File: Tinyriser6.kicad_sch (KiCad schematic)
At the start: 21 parts, among them J1 Bus_M.2_Socket_M, J2 Bus_PCI_Express_x16, J3 Conn_02x04_Odd_Even, J6 USB_A, J7 Conn_01x26_Pin, M1 Fan_4pin

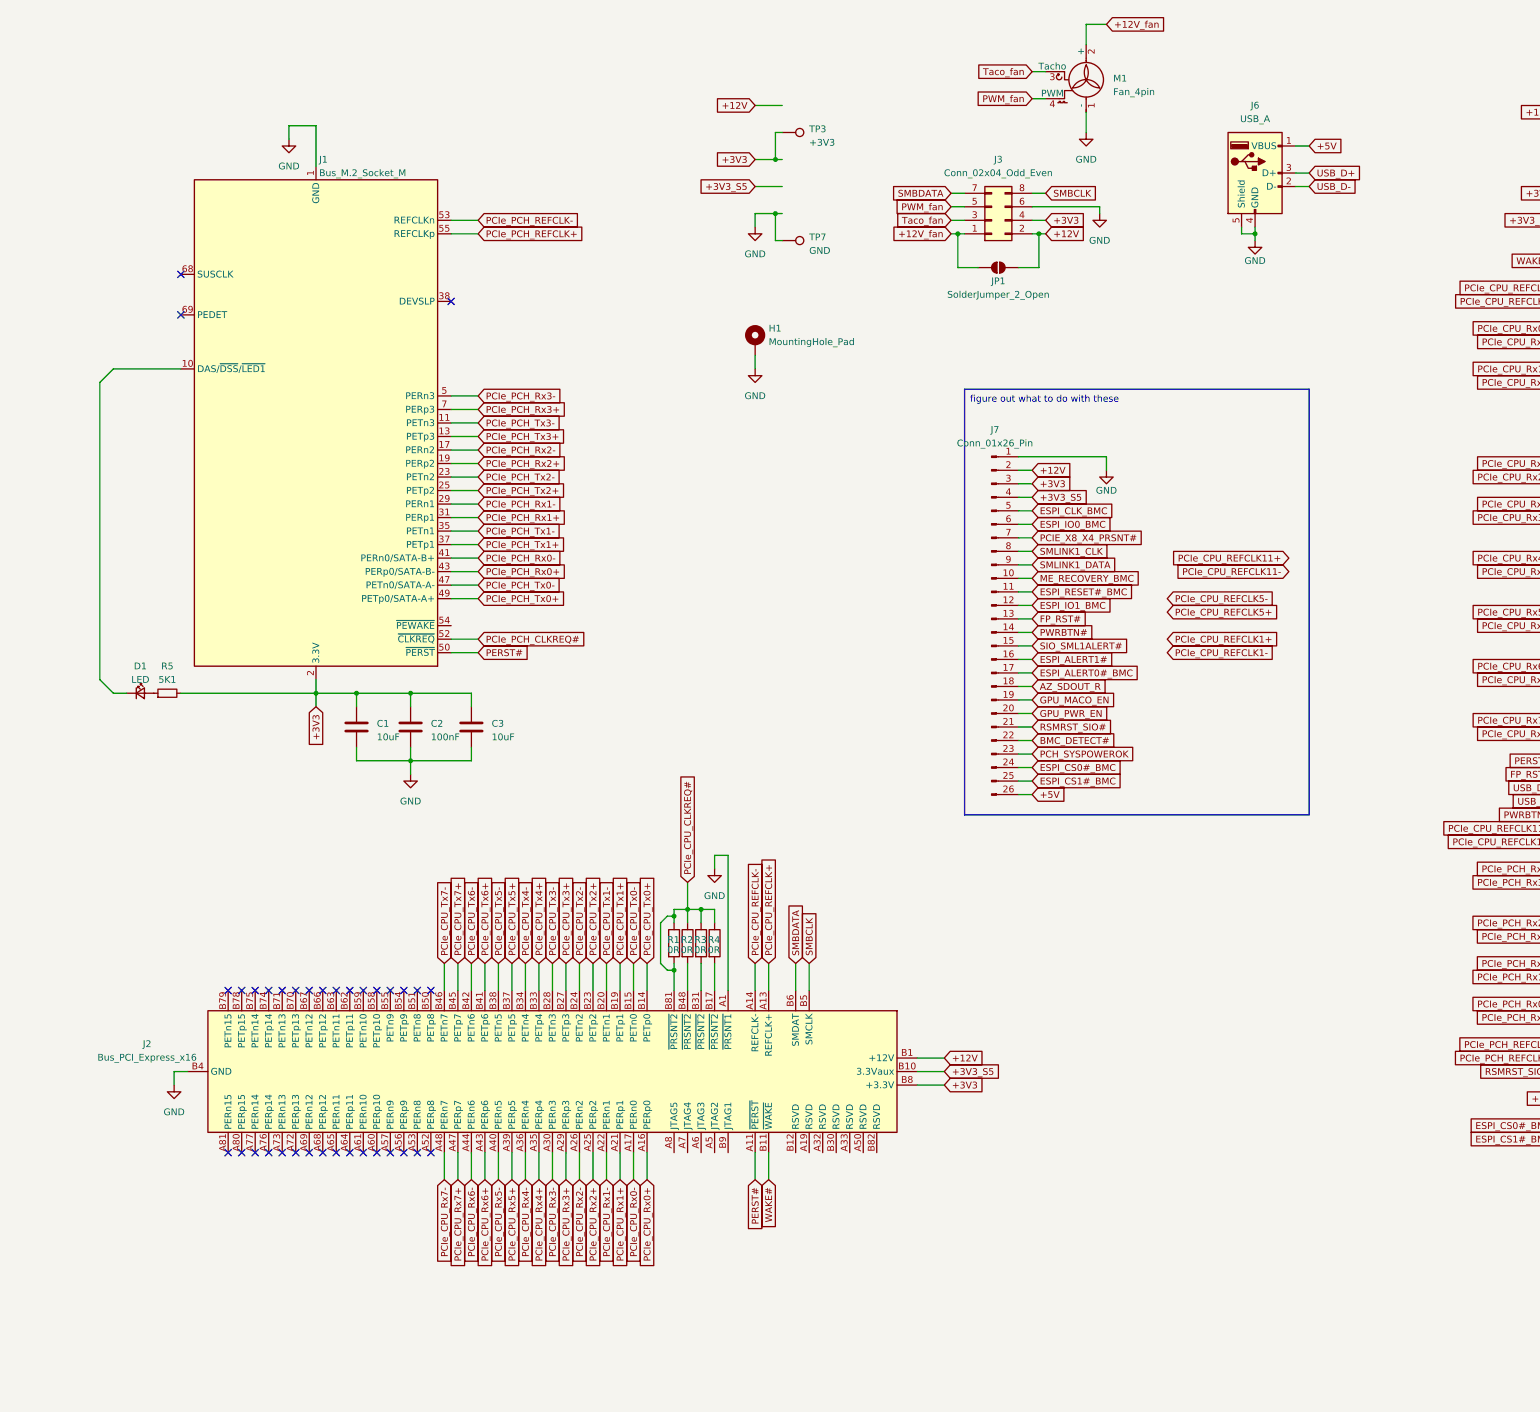
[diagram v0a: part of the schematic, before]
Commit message: Trying to figure out what to do with the random io
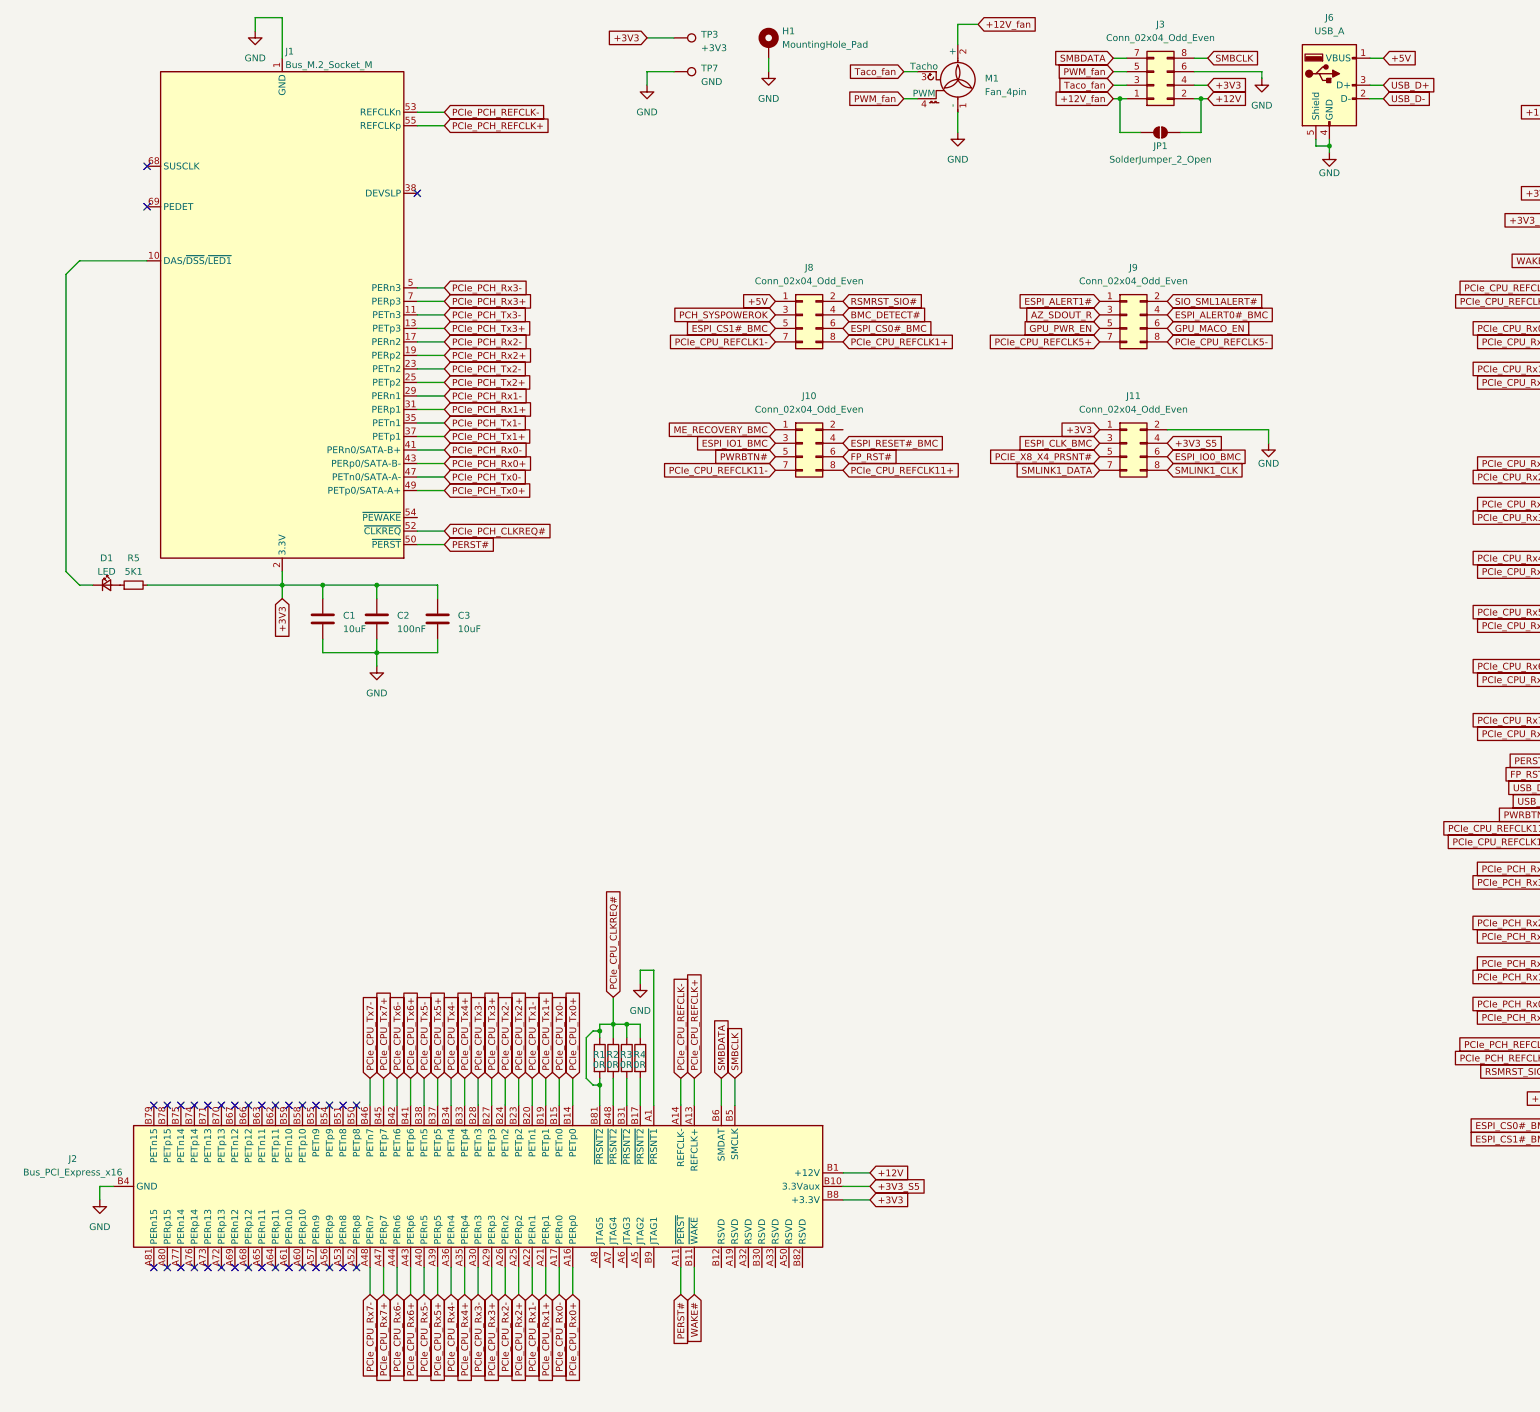
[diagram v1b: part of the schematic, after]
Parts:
- removed J7: Conn_01x26_Pin, Connector_PinHeader_2.00mm:PinHeader_2x13_P2.00mm_Vertical, symbol Connector:Conn_01x26_Pin
- added J10, J11, J8, J9: Conn_02x04_Odd_Even, Connector_PinHeader_2.00mm:PinHeader_2x04_P2.00mm_Vertical, symbol Connector_Generic:Conn_02x04_Odd_Even
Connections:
- net +3V3: now also J11.1 (Pin_1)
- net +3V3_S5: now also J11.4 (Pin_4)
- net +5V: now also J8.1 (Pin_1)
- net AZ_SDOUT_R: now also J9.3 (Pin_3)
- net BMC_DETECT#: now also J8.4 (Pin_4)
- net ESPI_ALERT0#_BMC: now also J9.4 (Pin_4)
- net ESPI_ALERT1#: now also J9.1 (Pin_1)
- net ESPI_CLK_BMC: now also J11.3 (Pin_3)
- net ESPI_CS0#_BMC: now also J8.6 (Pin_6)
- net ESPI_CS1#_BMC: now also J8.5 (Pin_5)
- net ESPI_IO0_BMC: now also J11.6 (Pin_6)
- net ESPI_IO1_BMC: now also J10.3 (Pin_3)
- net ESPI_RESET#_BMC: now also J10.4 (Pin_4)
- net FP_RST#: now also J10.6 (Pin_6)
- net GND: now also J11.2 (Pin_2)
- net GPU_MACO_EN: now also J9.6 (Pin_6)
- net GPU_PWR_EN: now also J9.5 (Pin_5)
- net ME_RECOVERY_BMC: now also J10.1 (Pin_1)
- net PCH_SYSPOWEROK: now also J8.3 (Pin_3)
- net PCIE_X8_X4_PRSNT#: now also J11.5 (Pin_5)
- net PCIe_CPU_REFCLK1+: now also J8.8 (Pin_8)
- net PCIe_CPU_REFCLK1-: now also J8.7 (Pin_7)
- net PCIe_CPU_REFCLK11+: now also J10.8 (Pin_8)
- net PCIe_CPU_REFCLK11-: now also J10.7 (Pin_7)
- net PCIe_CPU_REFCLK5+: now also J9.7 (Pin_7)
- net PCIe_CPU_REFCLK5-: now also J9.8 (Pin_8)
- net PWRBTN#: now also J10.5 (Pin_5)
- net RSMRST_SIO#: now also J8.2 (Pin_2)
- net SIO_SML1ALERT#: now also J9.2 (Pin_2)
- net SMLINK1_CLK: now also J11.8 (Pin_8)
- net SMLINK1_DATA: now also J11.7 (Pin_7)
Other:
- moved on the sheet: C1, C2, C3, D1, H1, J1, J2, J3, J6, JP1, M1, R1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
